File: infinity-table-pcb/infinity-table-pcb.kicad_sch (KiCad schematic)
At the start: 10 parts, among them J1 PJ-063AH, J2 Conn_01x05_Male, J3 Conn_01x10_Male

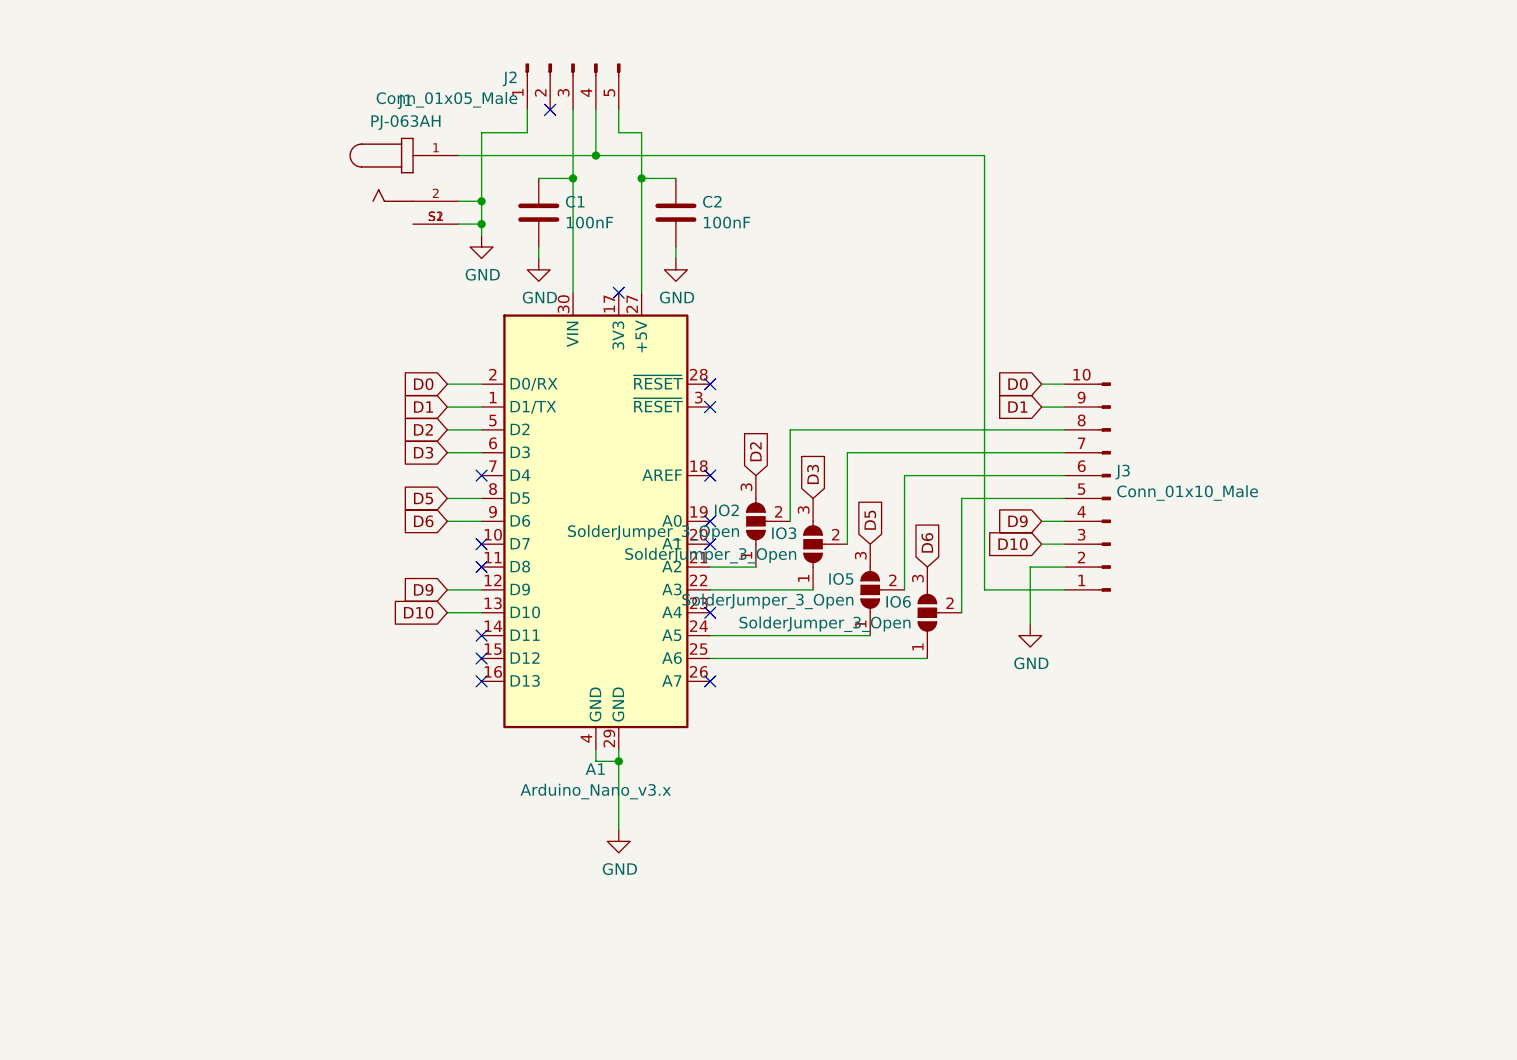
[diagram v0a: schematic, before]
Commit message: forgot to save work
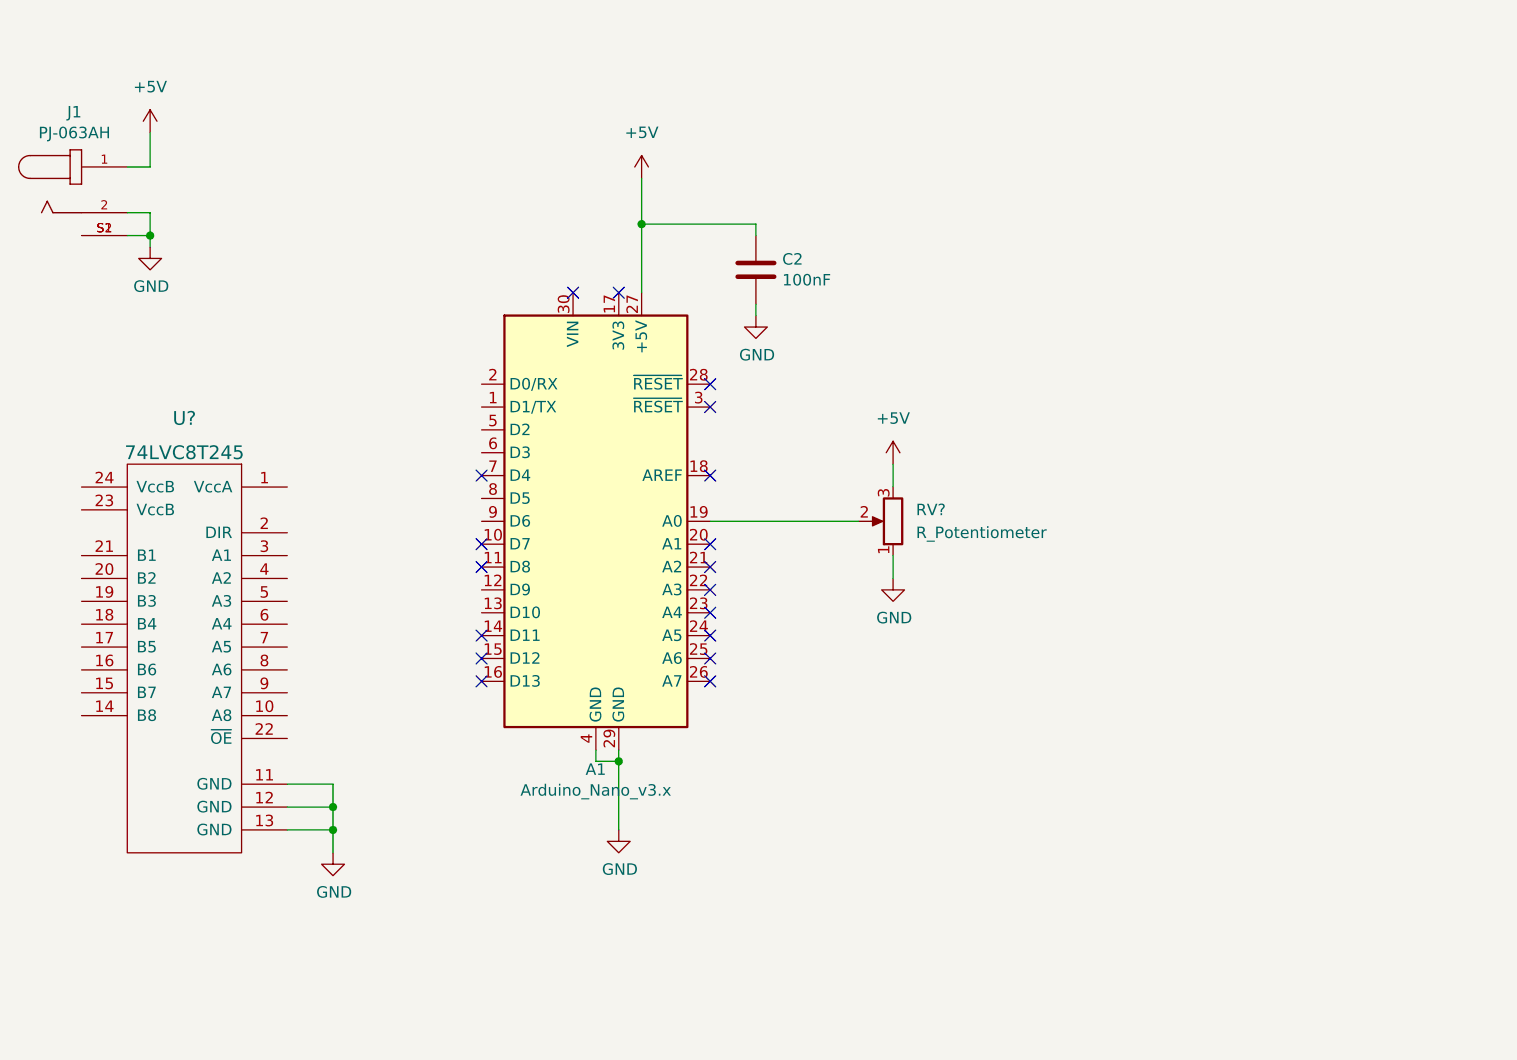
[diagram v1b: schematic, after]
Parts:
- removed C1: 100nF, Capacitor_SMD:C_0805_2012Metric, symbol Device:C
- removed IO2, IO3, IO5, IO6: SolderJumper_3_Open, Jumper:SolderJumper-3_P1.3mm_Open_Pad1.0x1.5mm, symbol Jumper:SolderJumper_3_Open
- removed J2: Conn_01x05_Male, Connector_PinHeader_2.54mm:PinHeader_1x05_P2.54mm_Vertical, symbol Connector:Conn_01x05_Male
- removed J3: Conn_01x10_Male, Connector_PinHeader_2.54mm:PinHeader_1x10_P2.54mm_Vertical, symbol Connector:Conn_01x10_Male
- added RV?: R_Potentiometer, symbol Device:R_Potentiometer
- added U?: 74LVC8T245, symbol 74LVC8T245:74LVC8T245
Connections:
- net GND: now also RV?.1, U?.11 (GND), U?.12 (GND), U?.13 (GND)
- net at A1.19 (A0): now also RV?.2
- net +5V: now reaches A1.27 (+5V), C2.1
- net +5V: now also J1.1, RV?.3
- net D0: no longer names the net of A1.2 (D0/RX)
- net D1: no longer names the net of A1.1 (D1/TX)
- net D10: no longer names the net of A1.13 (D10)
- net D2: no longer names the net of A1.5 (D2)
- net D3: no longer names the net of A1.6 (D3)
- net D5: no longer names the net of A1.8 (D5)
- net D6: no longer names the net of A1.9 (D6)
- net D9: no longer names the net of A1.12 (D9)
- no-connect marks 15 -> 18
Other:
- moved on the sheet: C2, J1

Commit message: wip infinity-table-pcb
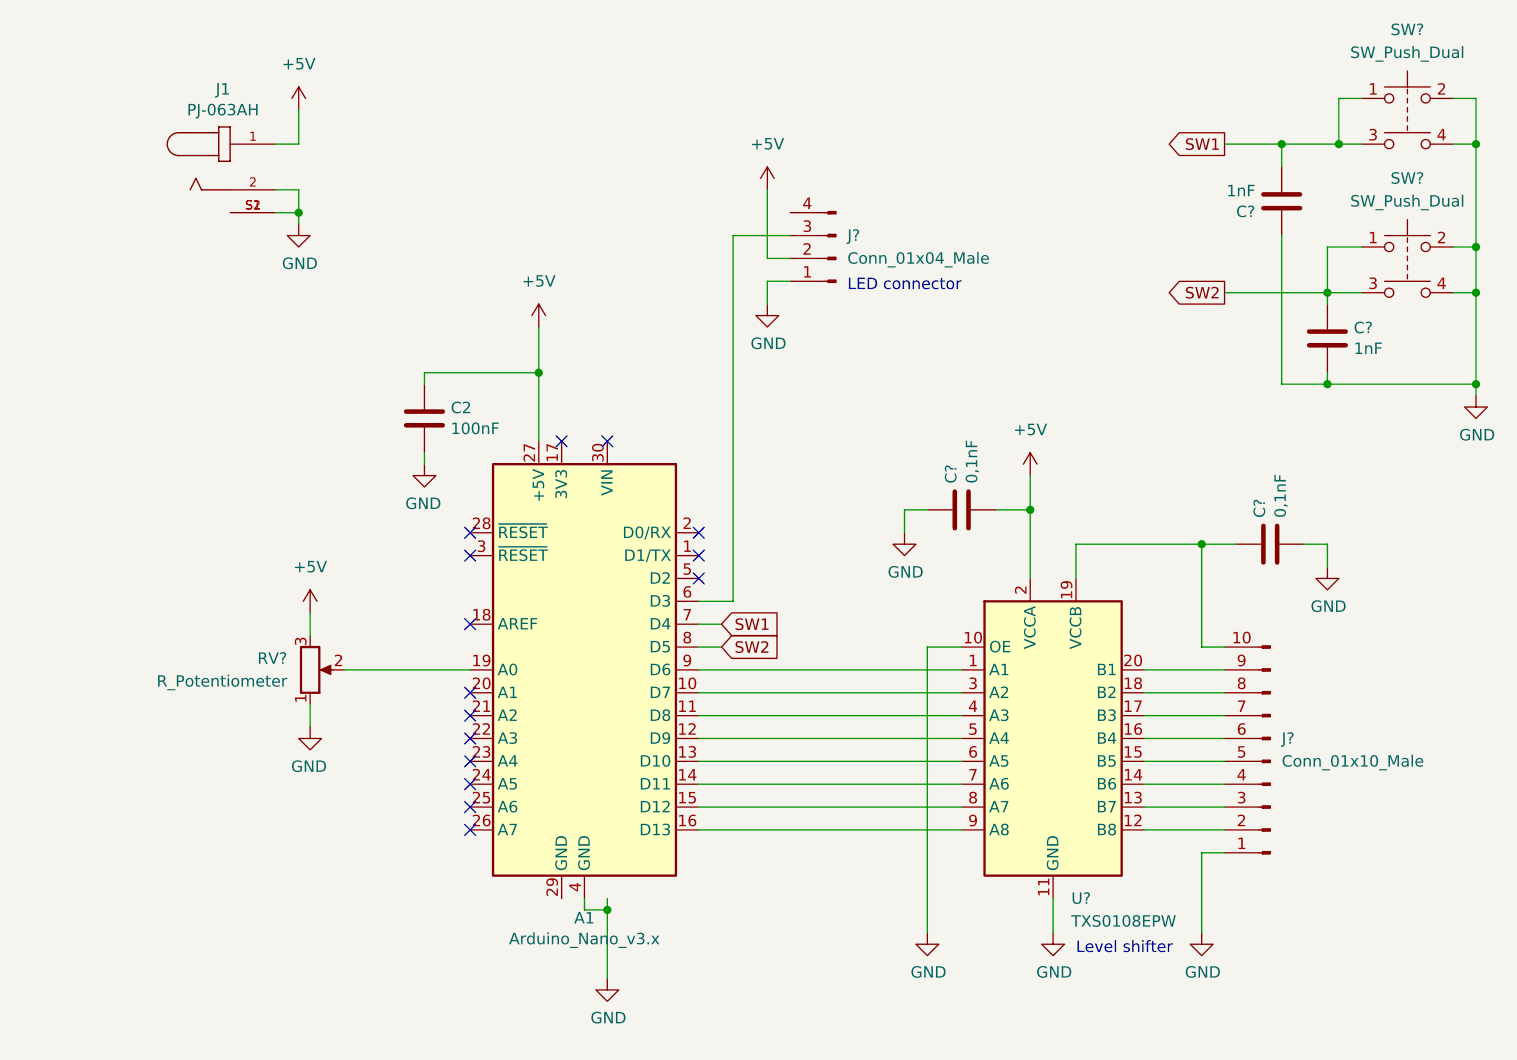
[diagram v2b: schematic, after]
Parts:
- removed U?: 74LVC8T245, symbol 74LVC8T245:74LVC8T245
- added C? (x2): 1nF, Capacitor_SMD:C_0805_2012Metric, symbol Device:C
- added C? (x2): 0,1nF, Capacitor_SMD:C_0805_2012Metric, symbol Device:C
- added J?: Conn_01x04_Male, symbol Connector:Conn_01x04_Male
- added J?: Conn_01x10_Male, symbol Connector:Conn_01x10_Male
- added SW? (x2): SW_Push_Dual, symbol Switch:SW_Push_Dual
- added U?: TXS0108EPW, Package_SO:TSSOP-20_4.4x6.5mm_P0.65mm, symbol Logic_LevelTranslator:TXS0108EPW
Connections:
- net +5V: now also C?.2, J?.2 (Pin_2), U?.2 (VCCA)
- net GND: now also C?.1, C?.1, C?.2, C?.2, J?.1 (Pin_1), J?.1 (Pin_1), SW?.2, SW?.2, SW?.4, SW?.4, U?.10 (OE), U?.11 (GND); no longer A1.29 (GND)
- net at A1.10 (D7): now also U?.3 (A2)
- net at A1.11 (D8): now also U?.4 (A3)
- net at A1.12 (D9): now also U?.5 (A4)
- net at A1.13 (D10): now also U?.6 (A5)
- net at A1.14 (D11): now also U?.7 (A6)
- net at A1.15 (D12): now also U?.8 (A7)
- net at A1.16 (D13): now also U?.9 (A8)
- net at A1.6 (D3): now also J?.3 (Pin_3)
- net SW1: now reaches A1.7 (D4)
- net SW1: now also C?.2, SW?.1, SW?.3
- net SW2: now reaches A1.8 (D5)
- net SW2: now also C?.1, SW?.1, SW?.3
- net at A1.9 (D6): now also U?.1 (A1)
- new net: J?.2 (Pin_2), U?.12 (B8)
- new net: J?.3 (Pin_3), U?.13 (B7)
- new net: J?.4 (Pin_4), U?.14 (B6)
- new net: J?.5 (Pin_5), U?.15 (B5)
- new net: J?.6 (Pin_6), U?.16 (B4)
- new net: J?.7 (Pin_7), U?.17 (B3)
- new net: J?.8 (Pin_8), U?.18 (B2)
- new net: C?.1, J?.10 (Pin_10), U?.19 (VCCB)
- new net: J?.9 (Pin_9), U?.20 (B1)
- no-connect marks 18 -> 15
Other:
- note added: "LED connector"
- note added: "Level shifter"
- moved on the sheet: A1, C2, J1, RV?

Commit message: pcb first version done, but need to rework a bit
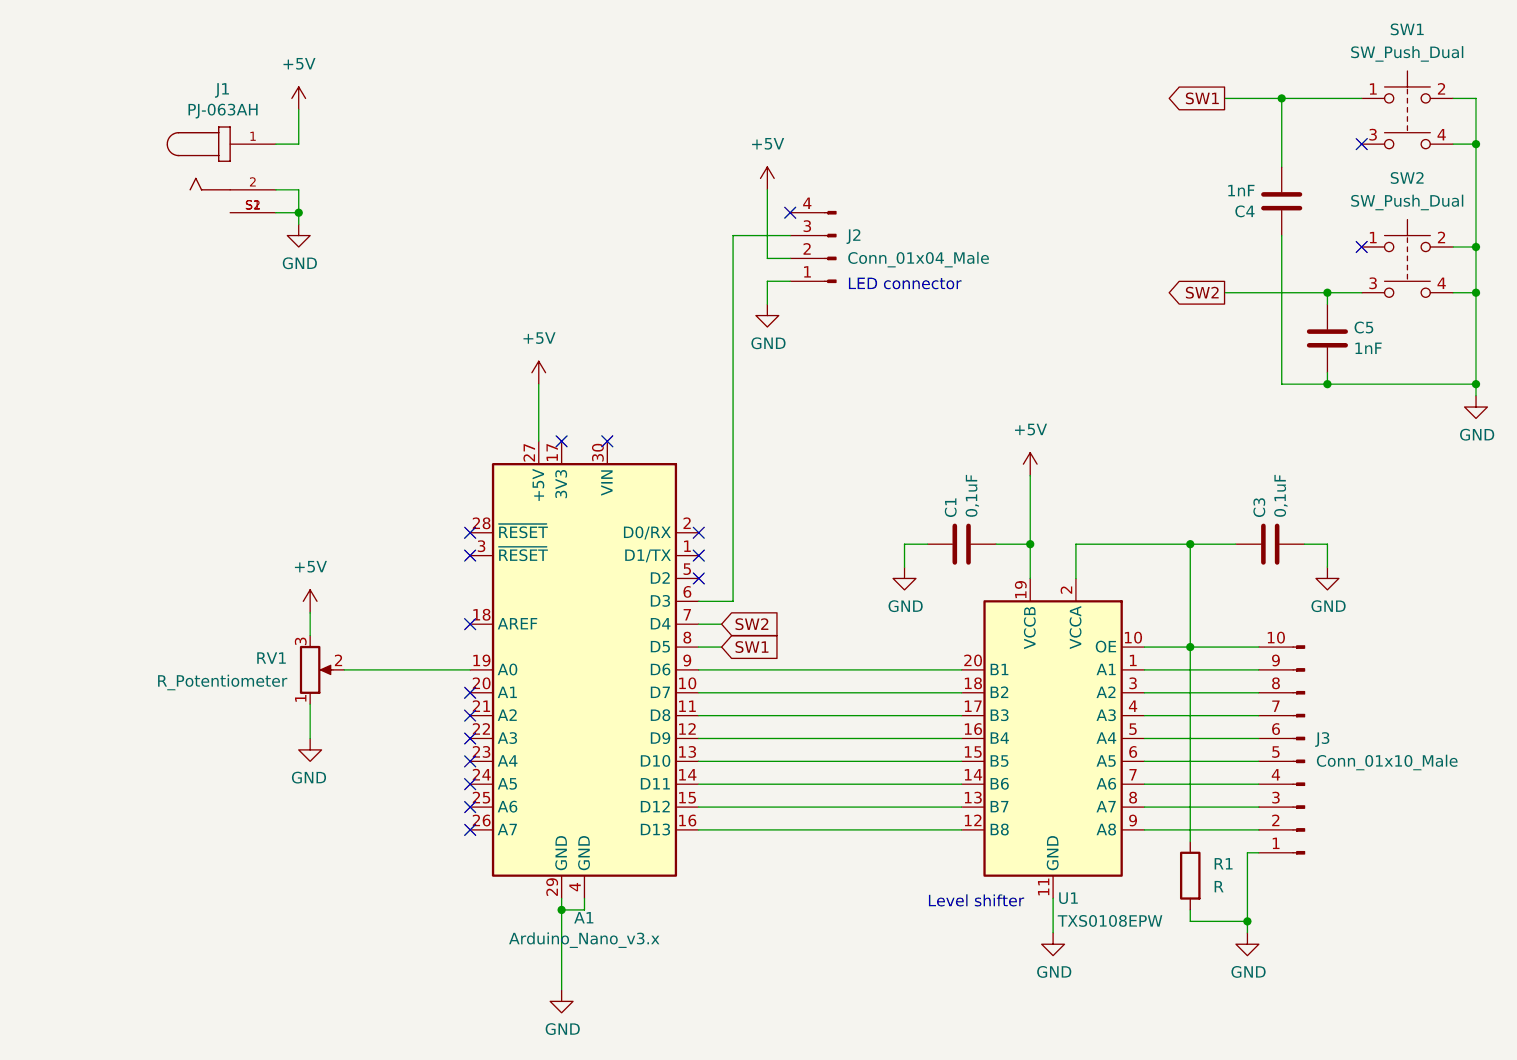
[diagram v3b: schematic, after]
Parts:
- removed C2: 100nF, Capacitor_SMD:C_0805_2012Metric, symbol Device:C
- added R1: R, Resistor_SMD:R_0805_2012Metric, symbol Device:R
- C1, C3: renamed from C?; value 0,1nF -> 0,1uF
- J1: footprint SS_connectors:CUI_PJ-063AH-1 -> kicad-ss-libs:CUI_PJ-063AH
- J2: renamed from J?; footprint (none) -> Connector_PinHeader_2.54mm:PinHeader_1x04_P2.54mm_Vertical
- J3: renamed from J?; footprint (none) -> Connector_PinHeader_2.54mm:PinHeader_1x10_P2.54mm_Vertical
- RV1: renamed from RV?; footprint (none) -> Connector_PinHeader_2.54mm:PinHeader_1x03_P2.54mm_Vertical
- SW1, SW2: renamed from SW?; footprint (none) -> kicad-ss-libs:Push Button 12x12mm
- gave numbers to parts that had none: 3
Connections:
- net +5V: now also U1.19 (VCCB); no longer U1.2 (VCCA)
- net GND: now also A1.29 (GND), R1.2; no longer U1.10 (OE)
- net SW1: now also A1.8 (D5); no longer A1.7 (D4), SW1.3
- net SW2: now also A1.7 (D4); no longer A1.8 (D5), SW2.1
- net at A1.10 (D7): now also U1.18 (B2); no longer U1.3 (A2)
- net at A1.11 (D8): now also U1.17 (B3); no longer U1.4 (A3)
- net at A1.12 (D9): now also U1.16 (B4); no longer U1.5 (A4)
- net at A1.13 (D10): now also U1.15 (B5); no longer U1.6 (A5)
- net at A1.14 (D11): now also U1.14 (B6); no longer U1.7 (A6)
- net at A1.15 (D12): now also U1.13 (B7); no longer U1.8 (A7)
- net at A1.16 (D13): now also U1.12 (B8); no longer U1.9 (A8)
- net at A1.9 (D6): now also U1.20 (B1); no longer U1.1 (A1)
- net at J3.2 (Pin_2): now also U1.9 (A8); no longer U1.12 (B8)
- net at J3.3 (Pin_3): now also U1.8 (A7); no longer U1.13 (B7)
- net at J3.4 (Pin_4): now also U1.7 (A6); no longer U1.14 (B6)
- net at J3.5 (Pin_5): now also U1.6 (A5); no longer U1.15 (B5)
- net at J3.6 (Pin_6): now also U1.5 (A4); no longer U1.16 (B4)
- net at J3.7 (Pin_7): now also U1.4 (A3); no longer U1.17 (B3)
- net at J3.8 (Pin_8): now also U1.3 (A2); no longer U1.18 (B2)
- net at C3.1, J3.10 (Pin_10): now also U1.10 (OE), U1.2 (VCCA), R1.1; no longer U1.19 (VCCB)
- net at J3.9 (Pin_9): now also U1.1 (A1); no longer U1.20 (B1)
- no-connect marks 15 -> 18
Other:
- moved on the sheet: C1, J3
